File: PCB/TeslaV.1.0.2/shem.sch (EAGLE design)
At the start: 90 parts, among them IC1 HC-06, IC2 STM32F042F4, IC3 AMS1117, IC4 UCC27424, IC5 74LVC2G14, IC6 LM311D, IC7 TNY274, J1 FAN, Q1 IRF7389, Q2 IRF7389, Q3 FGH40N60SMD, Q4 FGH40N60SMD

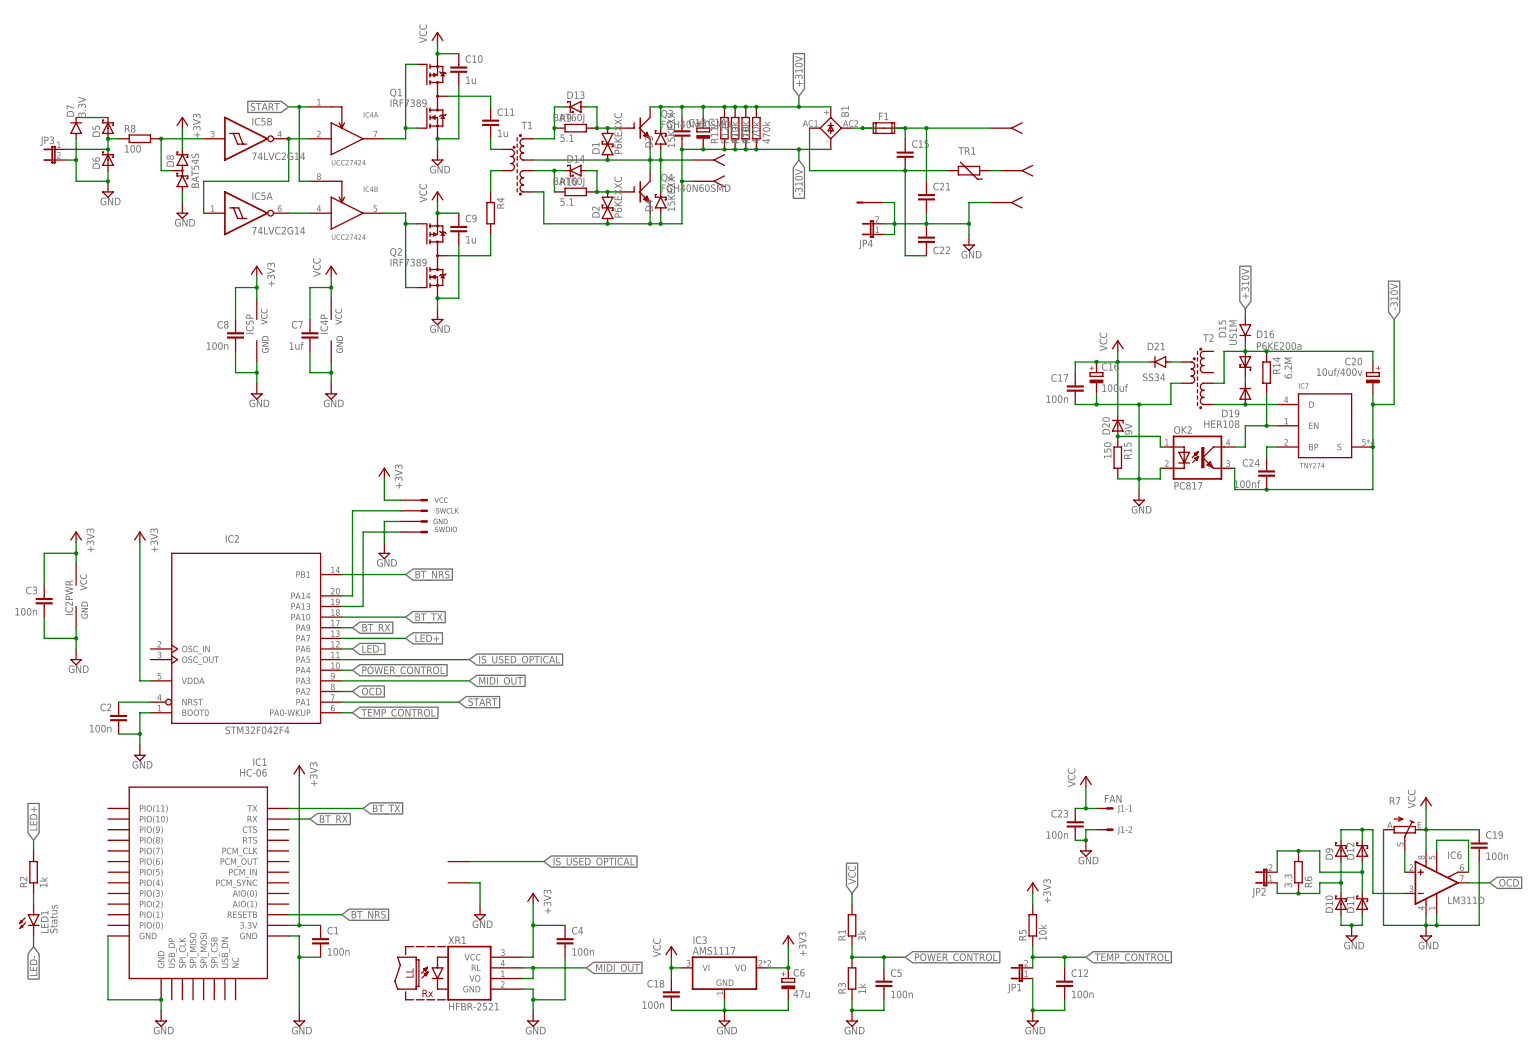
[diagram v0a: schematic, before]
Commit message: Release PCB
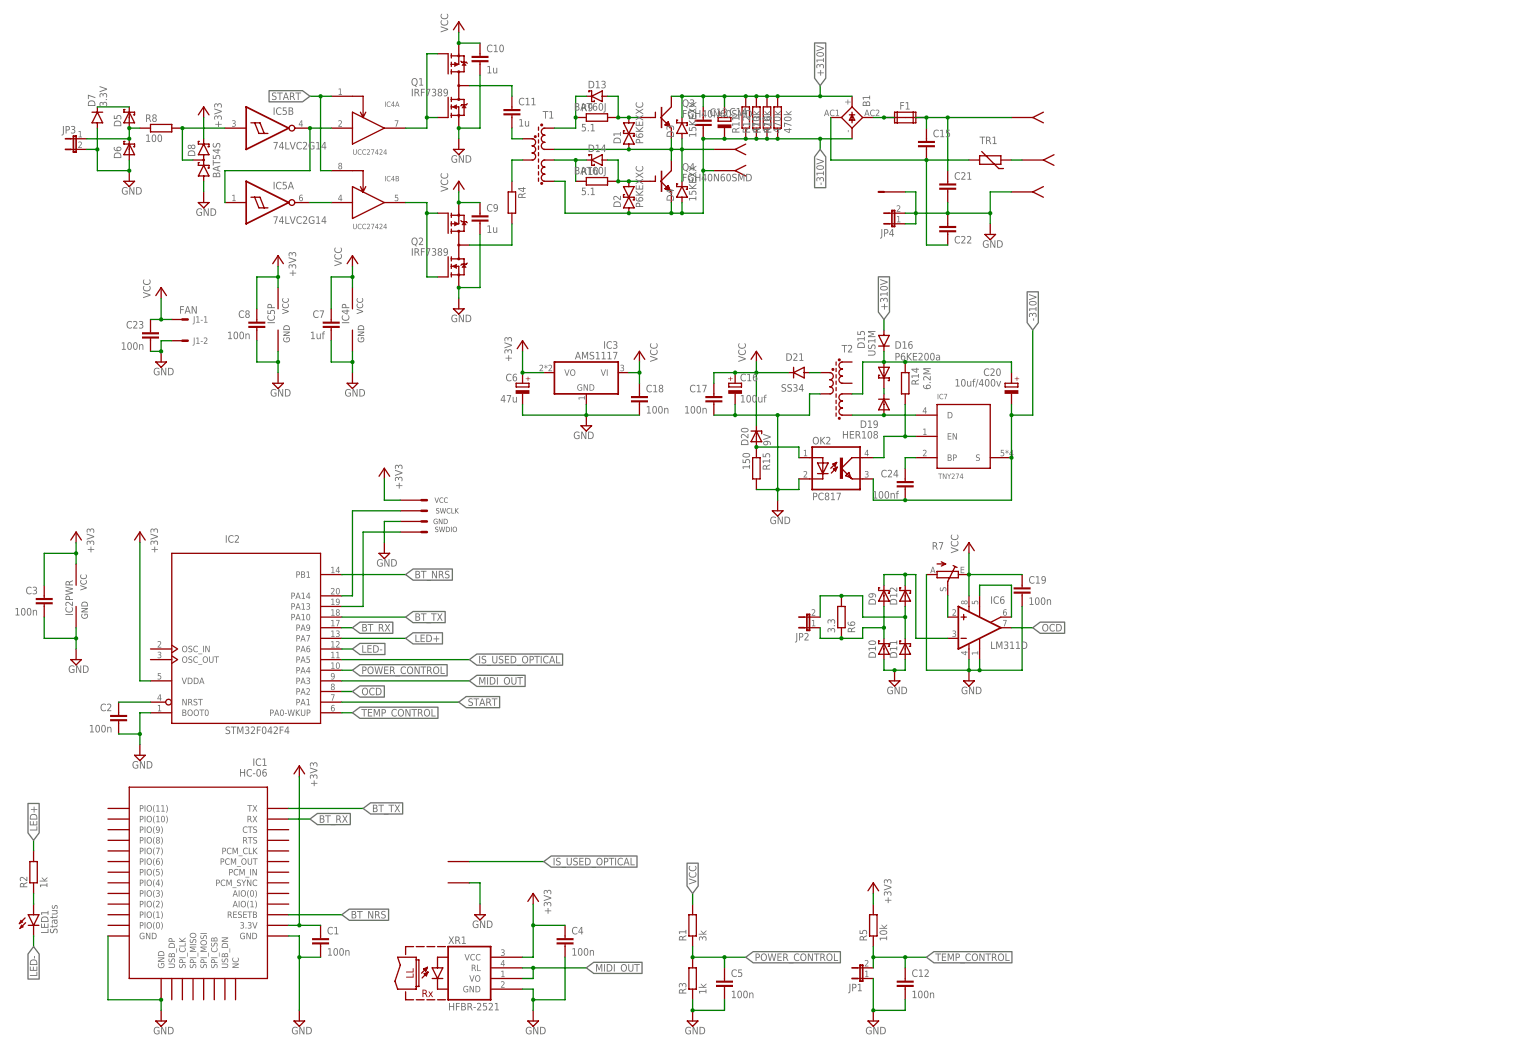
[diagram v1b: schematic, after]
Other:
- moved on the sheet: B1, C10, C11, C12, C13, C14, C15, C16, C17, C18, C19, C20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
